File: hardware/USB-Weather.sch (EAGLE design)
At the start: 84 parts, among them U1 ATMEGA328, U2 MIC5219-3.3BM5, U4 MCP73831, U5 HTU21DSMD, U6 TEMT6000, U7 BMP180, U8 FT231XS, Y1 8MHz

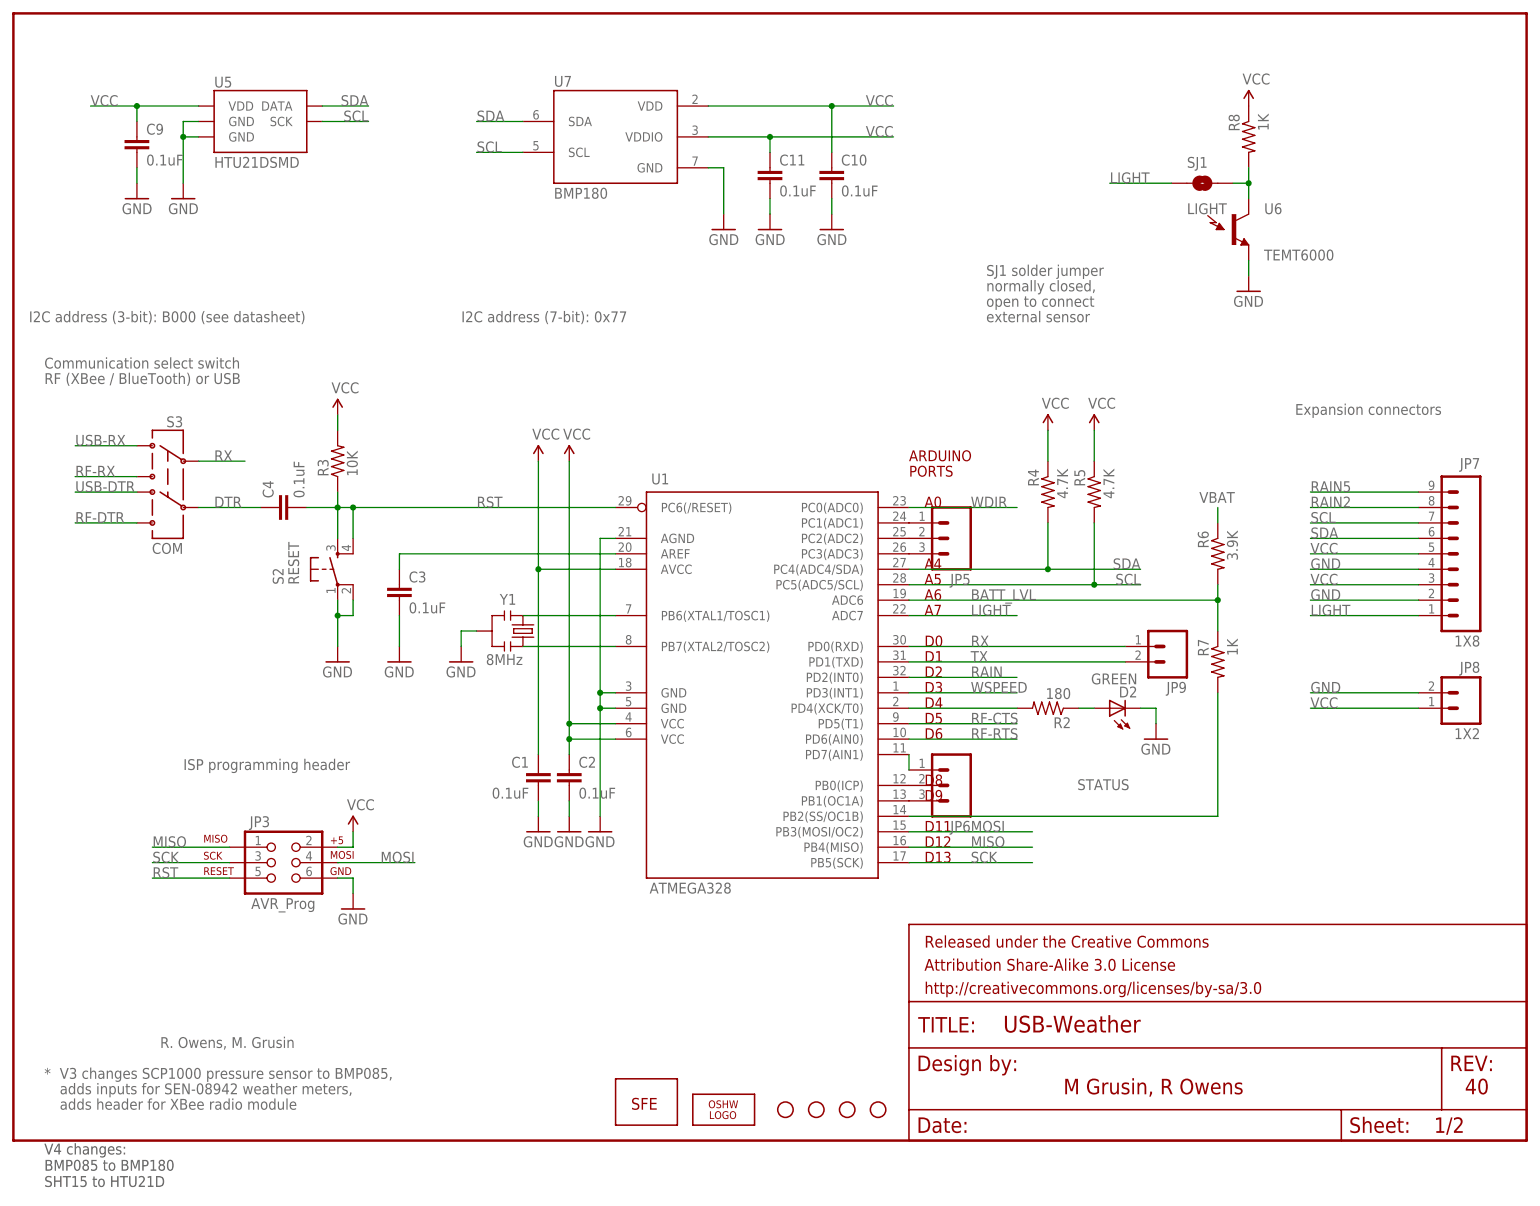
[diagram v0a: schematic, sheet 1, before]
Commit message: pre-review
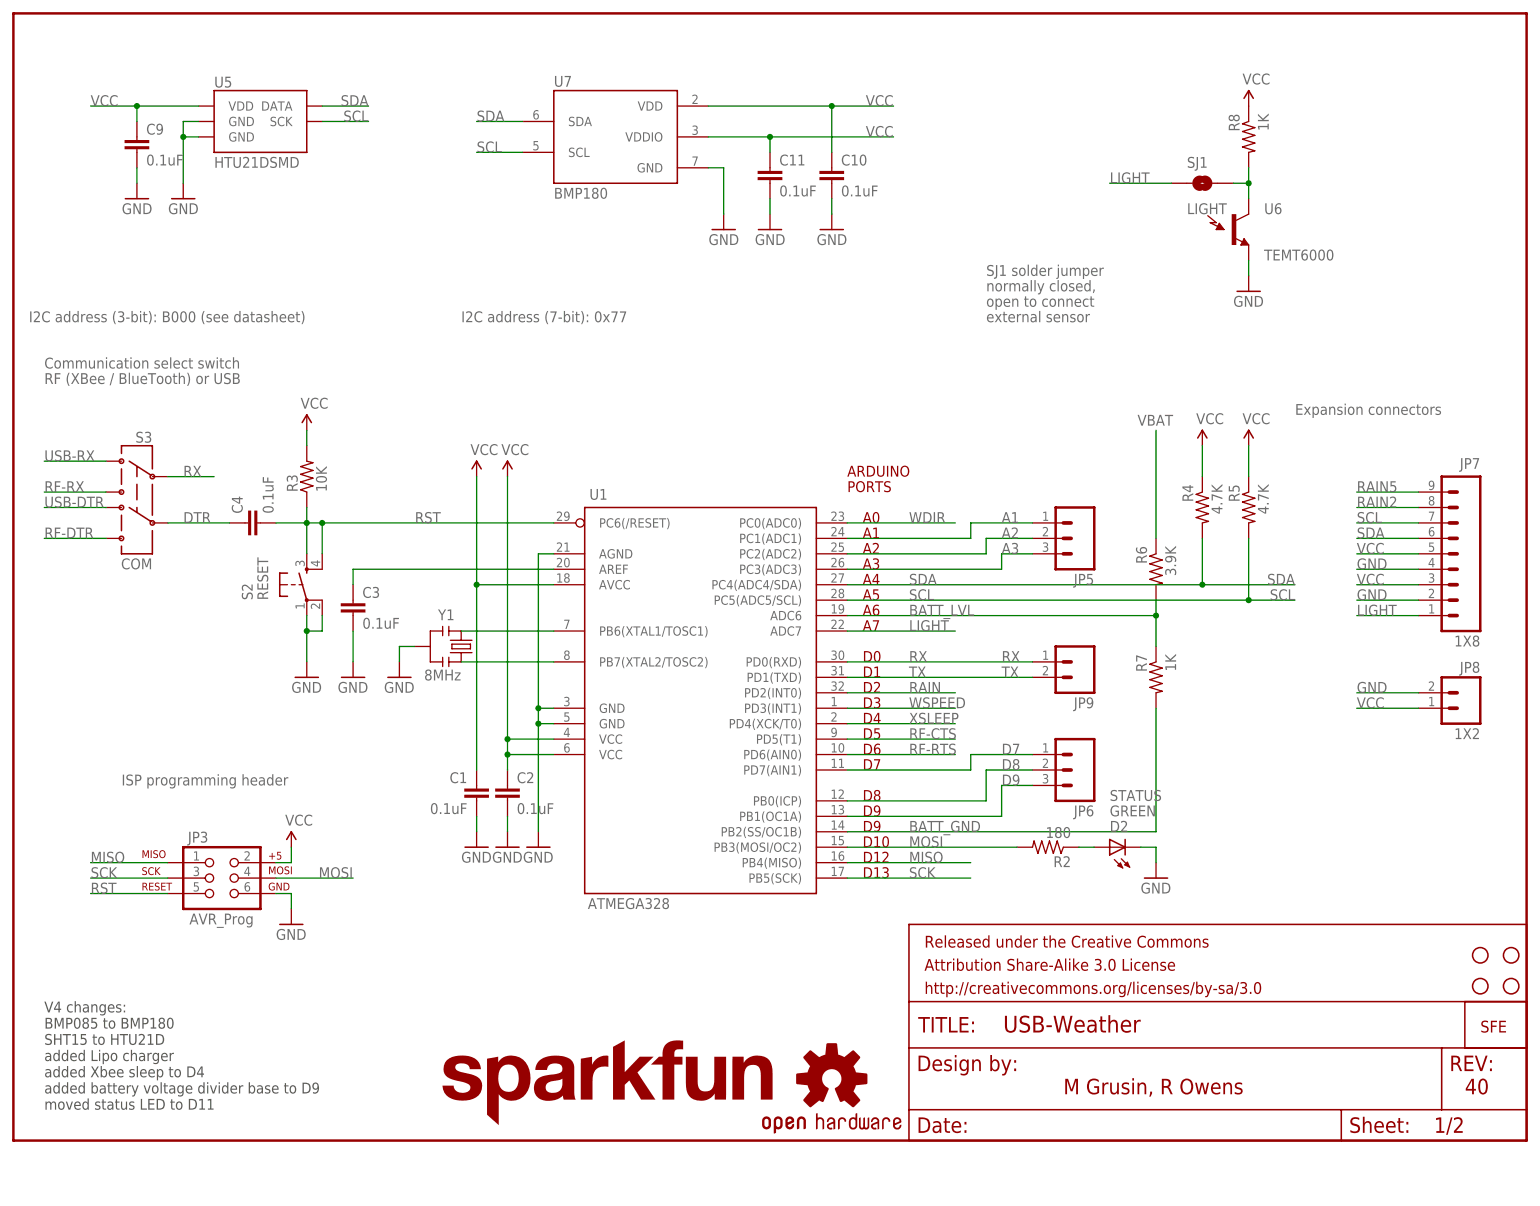
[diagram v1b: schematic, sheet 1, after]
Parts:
- removed C13: 4.7uF, SparkFun:CAP0603-CAP
- removed U$1: LOGO-SFENEW, SparkFun:LOGO-SFENEW
- added D13: BAS16, SparkFun:DIODESOD
- added LOGO2: OSHW-LOGOS, SparkFun-Aesthetics:OSHW-LOGOS
- added LOGO3: SFE_LOGO_NAME.1_INCH, SparkFun-Aesthetics:SFE_LOGO_NAME.1_INCH
- added R23: 10K, SparkFun:RESISTOR0603-RES
- D12: value RED -> YELLOW
- JP8: device SparkFun:M02PTH -> mike-temp:M021X02_NO_SILK
- LOGO1: value OSHW_LOGO_FILLX0100-NT -> LOGO-SFENEW; device OSHW:OSHW_LOGO_FILLX0100-NT -> SparkFun-Aesthetics:LOGO-SFENEW
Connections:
- net 3V-INT renamed N$26
- net N$15 renamed A1
- net N$16 renamed A2
- net N$17 renamed A3
- net N$18 renamed D8
- net N$19 renamed D9
- net N$20 renamed BATT_GND
- net N$21 renamed D7
- removed net N$4: R2.2, U1.PD4(XCK/T0)
- new net N$25: D13.A, JP4.VBUS, U8.VCC
- new net XSLEEP: JP6-DNP.DTR, R23.2, U1.PD4(XCK/T0)
- net GND: now also JP10.1; no longer C13.2, JP10.2
- net MOSI: now also R2.2
- net VBAT: now also S1.O; no longer S1.S
- net VCC: now also R23.1
- net VUSB: now also D13.C, JP10.2; no longer C13.1, JP10.1, JP4.VBUS, S1.O, U8.VCC
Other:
- note added: "A1"
- note added: "A2"
- note added: "A3"
- note added: "CHARGE"
- note added: "D10"
- note added: "D7"
- note added: "Lipo Charger"
- note added: "Pressure"
- note added: "V4 changes: BMP085 to BMP180 SHT15 to HTU21D added Lipo charger added Xbee sleep to D4 added battery voltage divider base to D9 moved status LED to D11"
- note removed: "*"
- note removed: "D11"
- note removed: "Power switch selects either"
- note removed: "Pressure*"
- note removed: "R. Owens, M. Grusin"
- note removed: "V3 changes SCP1000 pressure sensor to BMP085,"
- note removed: "V4 changes: BMP085 to BMP180 SHT15 to HTU21D"
- note removed: "adds header for XBee radio module"
- note removed: "adds inputs for SEN-08942 weather meters,"
- moved on the sheet: C1, C12, C14, C15, C2, C3, C4, C5, C6, C7, C8, D1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
